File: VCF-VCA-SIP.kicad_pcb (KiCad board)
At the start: 2 copper layers, 46 x 18 mm, 45 parts, among them P1 CONN_10, Q1 BC857BS, U1 LM13700, U2 TL072-, U3 LM13700, U4 TL072-, U5 LM13700, U6 TL072-

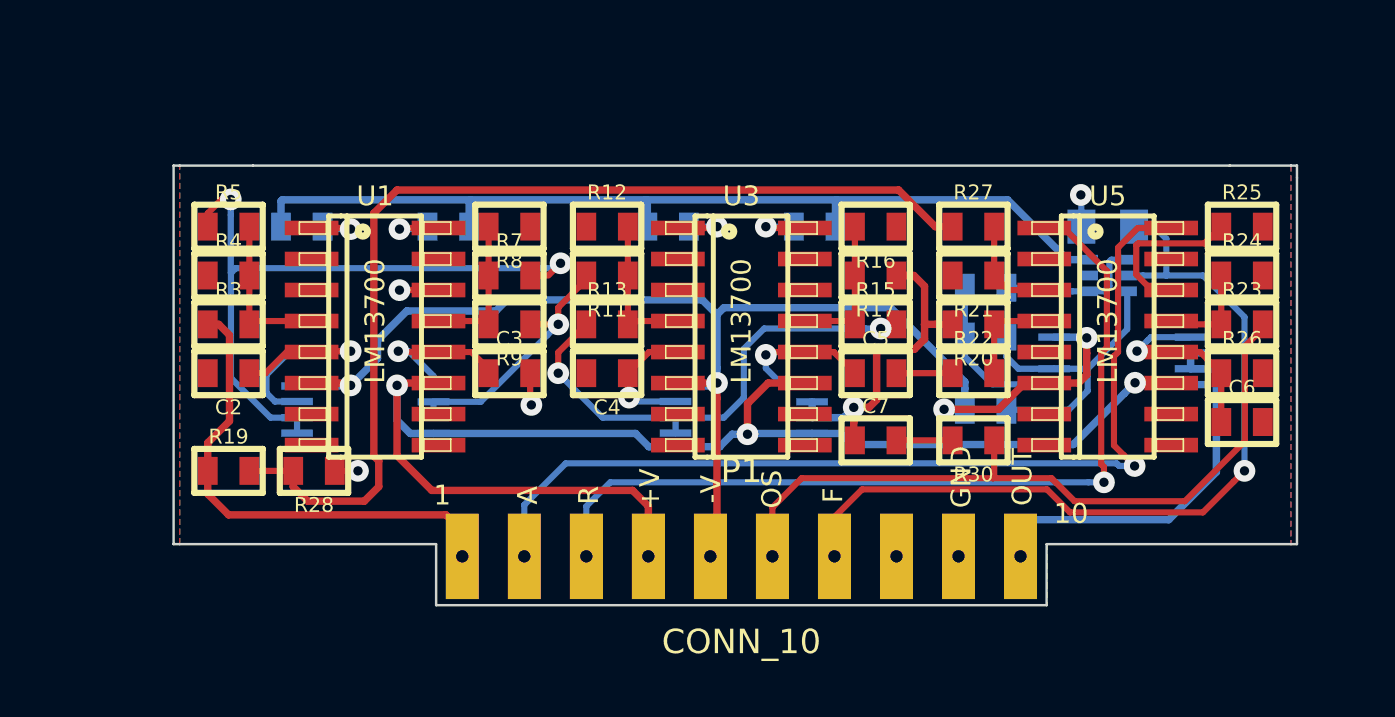
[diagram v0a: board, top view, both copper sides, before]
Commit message: rearrange components and reroute
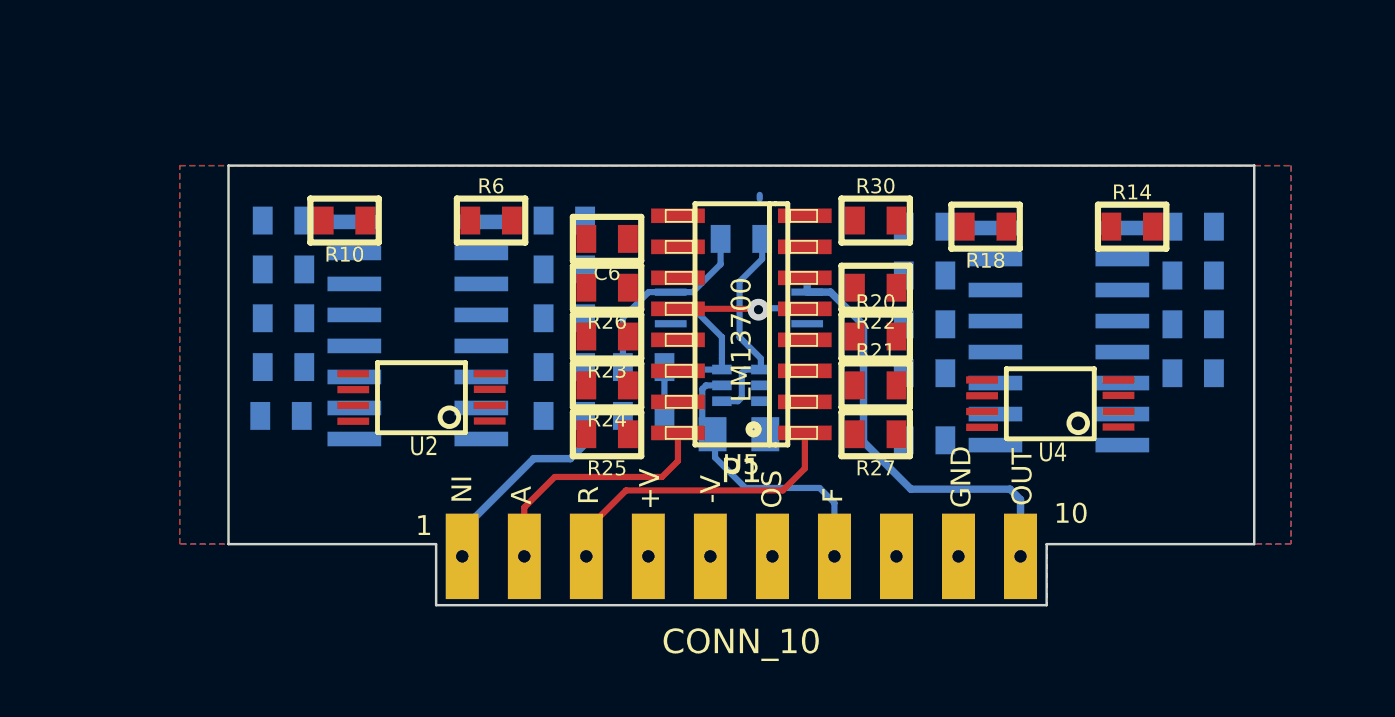
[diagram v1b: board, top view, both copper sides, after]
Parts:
- C2, C3, C4, C5, C7, R11, R12, R13, R15, R16, R17, R19, R28, R3, R4, R5, R7, R8, R9, U1, U3: moved to B.Cu
- R10, R14, R18, R6, U2, U4: moved to F.Cu
- moved R25 27.4 mm to (112.5, 94.0), turned to 180 degrees
- moved C6 27.1 mm to (112.5, 86.0), turned to 180 degrees
- moved R24 26.4 mm to (112.5, 92.0), turned to 180 degrees
- moved R26 26.2 mm to (112.5, 88.0), turned to 180 degrees
- moved R23 26.0 mm to (112.5, 90.0), turned to 180 degrees
- moved C4 24.0 mm to (136.5, 91.5), turned to 0 degrees
- moved R11 24.0 mm to (136.5, 87.5), turned to 0 degrees
- moved R12 24.0 mm to (136.5, 85.5), turned to 180 degrees
- moved R13 24.0 mm to (136.5, 89.5), turned to 180 degrees
- moved R14 19.0 mm to (134.0, 85.5), turned to 0 degrees
- moved R29 17.3 mm to (117.9, 94.0), turned to 0 degrees
- moved U6 15.7 mm to (118.0, 88.5), turned to 270 degrees
- moved Q1 15.7 mm to (118.0, 92.0), turned to 270 degrees
- moved U5 15.0 mm to (118.0, 89.5), turned to 90 degrees
- moved C1 14.1 mm to (114.0, 91.2)
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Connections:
- U6 pad 1: Net-(C1-Pad1) -> VCA_OUT
- U6 pad 2: Net-(C1-Pad2) -> VCA_OUT
- U6 pad 3: GND -> Net-(C6-Pad1)
- U6 pad 5: Net-(C6-Pad1) -> GND
- U6 pad 6: VCA_OUT -> Net-(C1-Pad2)
- U6 pad 7: VCA_OUT -> Net-(C1-Pad1)
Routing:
- net +VCC: track 60.6 -> 0.00 mm, vias 3 -> 0
- net -VCC: track 57.1 -> 0.00 mm, vias 4 -> 0
- net Net-(R19-Pad2): track 42.6 -> 0.00 mm
- net Iabc: track 38.7 -> 0.00 mm
- net OFFSET: track 30.2 -> 0.00 mm
- net VCA_CTRL: track 39.7 -> 10.2 mm, vias 1 -> 0
- net Net-(R5-Pad1): track 28.1 -> 0.00 mm, vias 2 -> 0
- net RES_CTRL: track 35.7 -> 12.5 mm, vias 1 -> 0
- net VCF_CTRL: track 34.8 -> 12.4 mm, vias 1 -> 0
- net Net-(R13-Pad1): track 20.6 -> 0.00 mm, vias 2 -> 0
- net VCF_OUT: track 14.1 -> 0.00 mm, vias 1 -> 0
- net VCF_IN: track 20.2 -> 8.72 mm
- net Net-(C2-Pad1): track 10.9 -> 0.00 mm, vias 1 -> 0
- net Net-(R11-Pad2): track 10.7 -> 0.00 mm, vias 1 -> 0
- net GND: track 7.48 -> 0.00 mm, vias 4 -> 0
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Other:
- board size 46 x 18 mm -> 42 x 18 mm

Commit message: probably going to give up on this layout. What a pain
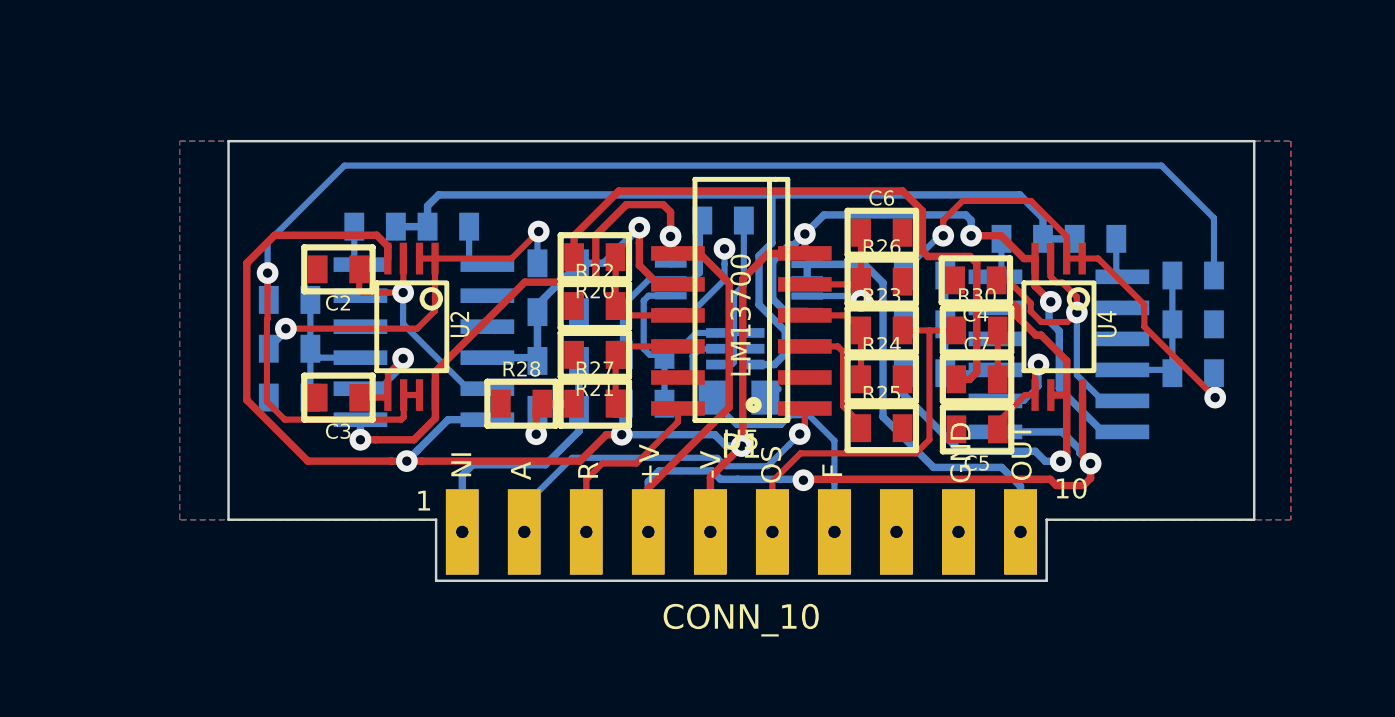
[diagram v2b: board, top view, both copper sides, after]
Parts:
- C2, C3, C4, C5, C7, R28: moved to F.Cu
- R10, R14, R18, R6: moved to B.Cu
- U1, U3, U5: footprint MyModules:SO16-JRL -> MyModules:SOIC16-12-JRL
- moved R20 12.0 mm to (112.0, 86.8), turned to 180 degrees
- moved R21 11.6 mm to (112.0, 90.8), turned to 180 degrees
- moved R27 11.6 mm to (112.0, 92.8), turned to 0 degrees
- moved R22 11.5 mm to (112.0, 88.8), turned to 0 degrees
- moved C6 11.3 mm to (123.8, 85.8), turned to 0 degrees
- moved R23 11.3 mm to (123.8, 89.8), turned to 0 degrees
- moved R24 11.3 mm to (123.8, 91.8), turned to 0 degrees
- moved R25 11.3 mm to (123.8, 93.8), turned to 0 degrees
- moved R26 11.3 mm to (123.8, 87.8), turned to 0 degrees
- moved C2 10.1 mm to (101.5, 87.2), turned to 180 degrees
- moved R28 9.86 mm to (109.0, 92.8)
- moved C4 9.68 mm to (127.6, 87.7), turned to 180 degrees
- moved R8 7.25 mm to (99.5, 92.5)
- moved R30 6.12 mm to (127.6, 89.8)
- moved R12 4.00 mm to (136.5, 89.5)
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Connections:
- U5 pad 1: RES_CTRL -> VCA_CTRL
- U5 pad 12: Net-(C6-Pad1) -> Net-(R3-Pad2)
- U5 pad 13: Net-(R23-Pad1) -> Net-(R20-Pad1)
- U5 pad 14: Net-(R25-Pad1) -> Net-(R21-Pad1)
- U5 pad 16: VCA_CTRL -> RES_CTRL
- U5 pad 3: Net-(R21-Pad1) -> Net-(R25-Pad1)
- U5 pad 4: Net-(R20-Pad1) -> Net-(R23-Pad1)
- U5 pad 5: Net-(R3-Pad2) -> Net-(C6-Pad1)
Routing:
- net -VCC: track 0.00 -> 81.4 mm, vias 0 -> 6
- net +VCC: track 0.00 -> 66.8 mm, vias 0 -> 4
- net Net-(R11-Pad2): track 0.00 -> 58.4 mm, vias 0 -> 1
- net VCF_OUT: track 0.00 -> 43.9 mm, vias 0 -> 1
- net Iabc: track 0.00 -> 38.4 mm
- net Net-(R13-Pad1): track 0.00 -> 19.9 mm, vias 0 -> 2
- net Net-(R5-Pad1): track 0.00 -> 16.3 mm, vias 0 -> 2
- net OFFSET: track 0.00 -> 15.9 mm
- net Net-(R3-Pad2): track 0.00 -> 13.3 mm, vias 0 -> 1
- net Net-(C4-Pad1): track 0.00 -> 12.0 mm, vias 0 -> 1
- net Net-(C2-Pad1): track 0.00 -> 9.91 mm, vias 0 -> 1
- net VCA_CTRL: track 10.2 -> 17.0 mm, vias 0 -> 1
- net Net-(C5-Pad1): track 0.00 -> 6.49 mm, vias 0 -> 1
- net Net-(R7-Pad1): track 0.00 -> 6.20 mm
- net Net-(R15-Pad1): track 0.00 -> 6.11 mm
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
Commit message: still struggling. about to go back to original layout
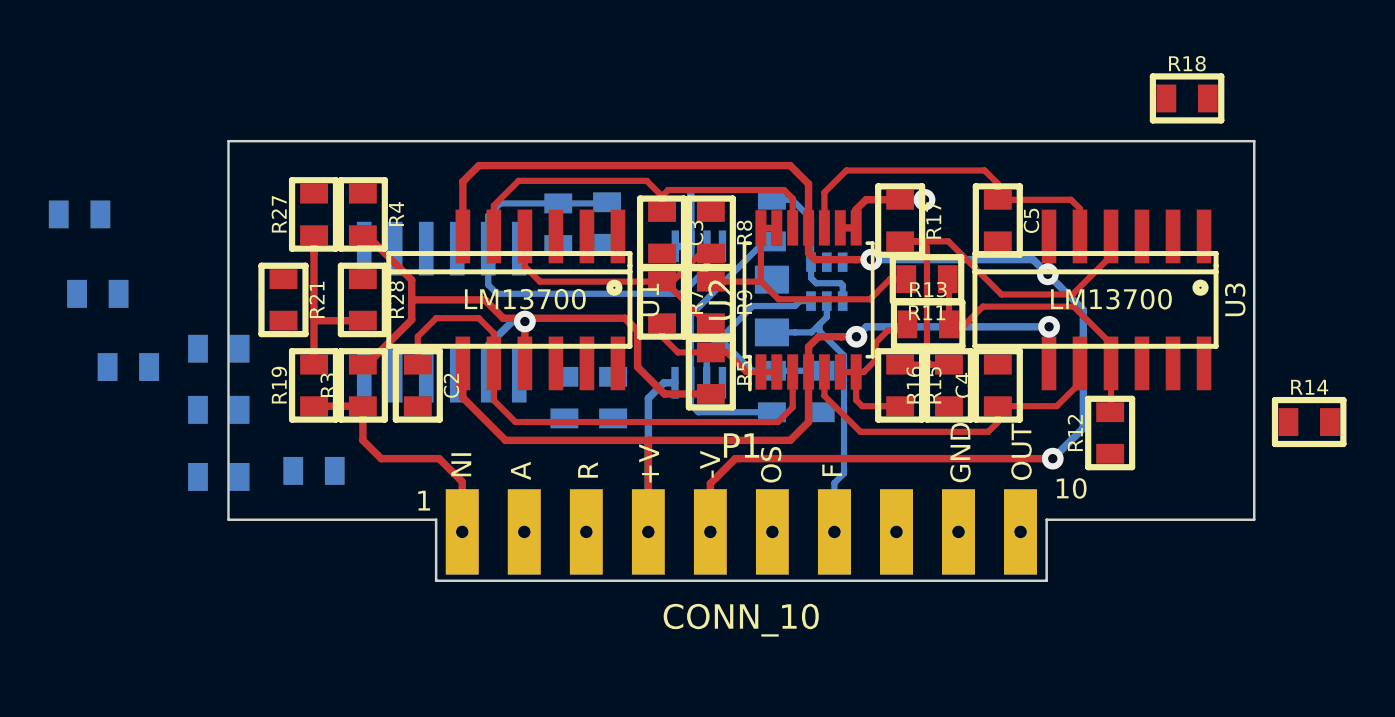
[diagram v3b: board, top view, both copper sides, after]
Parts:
- removed U6: TL072-, MyModules:TSSOP8-JRL
- C6, C7, R20, R22, R23, R24, R25, R26, R30: moved to B.Cu
- R11, R12, R13, R14, R15, R16, R17, R18, R19, R3, R4, R5, R7, R8, R9, U1, U3: moved to F.Cu
- U2: value TL072- -> TL074-; footprint MyModules:TSSOP8-JRL -> Housings_SSOP:TSSOP-14_4.4x5mm_Pitch0.65mm
- U4: value TL072- -> LM13700; footprint MyModules:TSSOP8-JRL -> MyModules:SOIC16-12-JRL; moved to B.Cu
- U5: value LM13700 -> TL072-; footprint MyModules:SOIC16-12-JRL -> MyModules:TSSOP8-JRL; moved to B.Cu
- moved R24 33.5 mm to (90.9, 85.0)
- moved R25 32.6 mm to (91.6, 88.2)
- moved C7 31.1 mm to (96.6, 93.0)
- moved R30 31.1 mm to (96.6, 90.5)
- moved R23 30.9 mm to (92.9, 91.2)
- moved U4 24.0 mm to (107.0, 89.0), turned to 0 degrees
- moved R8 18.5 mm to (116.8, 85.8), turned to 270 degrees
- moved R20 17.8 mm to (96.6, 95.8)
- moved R9 17.3 mm to (116.8, 88.6), turned to 270 degrees
- moved U2 16.3 mm to (120.8, 88.5), turned to 90 degrees
- moved R7 15.4 mm to (114.8, 88.6), turned to 270 degrees
- moved C3 14.9 mm to (114.8, 85.8), turned to 270 degrees
- moved R27 13.9 mm to (100.5, 85.0), turned to 90 degrees
- moved R26 13.5 mm to (110.5, 85.4), turned to 270 degrees
- moved R22 13.3 mm to (100.5, 95.5)
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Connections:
- U1 pad 1: Net-(R6-Pad1) -> Net-(R10-Pad1)
- U1 pad 12: Net-(C3-Pad1) -> Net-(C2-Pad1)
- U1 pad 13: Net-(R7-Pad1) -> Net-(R3-Pad2)
- U1 pad 16: Net-(R10-Pad1) -> Net-(R6-Pad1)
- U1 pad 4: Net-(R3-Pad2) -> Net-(R7-Pad1)
- U1 pad 5: Net-(C2-Pad1) -> Net-(C3-Pad1)
- U2 pad 4: -VCC -> +VCC
- U2 pad 5: Net-(C3-Pad1) -> Net-(C4-Pad1)
- U2 pad 6: Net-(R11-Pad2) -> Net-(R13-Pad1)
- U2 pad 7: Net-(R11-Pad2) -> Net-(R13-Pad1)
- U2 pad 8: +VCC -> VCF_OUT
- U3 pad 1: Net-(R14-Pad1) -> Net-(R18-Pad1)
- U3 pad 12: Net-(C5-Pad1) -> Net-(C4-Pad1)
- U3 pad 13: Net-(R15-Pad1) -> Net-(R11-Pad1)
- U3 pad 16: Net-(R18-Pad1) -> Net-(R14-Pad1)
- U3 pad 4: Net-(R11-Pad1) -> Net-(R15-Pad1)
- U3 pad 5: Net-(C4-Pad1) -> Net-(C5-Pad1)
- U4 pad 1: Net-(R13-Pad1) -> VCA_CTRL
- U4 pad 2: Net-(R13-Pad1) -> Net-(U4-Pad2)
- U4 pad 3: Net-(C4-Pad1) -> Net-(R25-Pad1)
- U4 pad 4: -VCC -> Net-(R23-Pad1)
- U4 pad 5: Net-(C5-Pad1) -> Net-(C6-Pad1)
- U4 pad 6: VCF_OUT -> -VCC
- U5 pad 1: VCA_CTRL -> VCA_OUT
- U5 pad 2: Net-(U5-Pad2) -> VCA_OUT
- U5 pad 3: Net-(R25-Pad1) -> Net-(C6-Pad1)
- U5 pad 4: Net-(R23-Pad1) -> -VCC
- U5 pad 5: Net-(C6-Pad1) -> GND
- U5 pad 6: -VCC -> Net-(C1-Pad2)
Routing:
- net Net-(R11-Pad2): track 58.4 -> 11.6 mm, vias 1 -> 0
- net VCF_OUT: track 43.9 -> 4.37 mm
- net Iabc: track 38.4 -> 0.00 mm
- net +VCC: track 66.8 -> 42.0 mm, vias 4 -> 2
- net -VCC: track 81.4 -> 56.7 mm, vias 6 -> 3
- net VCA_CTRL: track 17.0 -> 0.00 mm, vias 1 -> 0
- net VCA_OUT: track 19.3 -> 2.87 mm
- net OFFSET: track 15.9 -> 0.00 mm
- net Net-(R3-Pad2): track 13.3 -> 26.9 mm
- net Net-(R15-Pad1): track 6.11 -> 19.1 mm
- net Net-(R13-Pad1): track 19.9 -> 7.12 mm, vias 2 -> 0
- net Net-(C2-Pad1): track 9.91 -> 21.9 mm, vias 1 -> 0
- net Net-(C6-Pad1): track 7.41 -> 18.4 mm, vias 1 -> 0
- net Net-(C3-Pad1): track 5.40 -> 16.3 mm, vias 1 -> 0
- net RES_CTRL: track 10.5 -> 0.00 mm
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- removed copper zone on B.Cu, net GND
- removed copper zone on F.Cu, net GND
